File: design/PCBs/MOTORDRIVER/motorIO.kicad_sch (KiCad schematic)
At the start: 3 parts, among them J5 1-84952-1, J6 1-84952-1, J7 1-84952-1

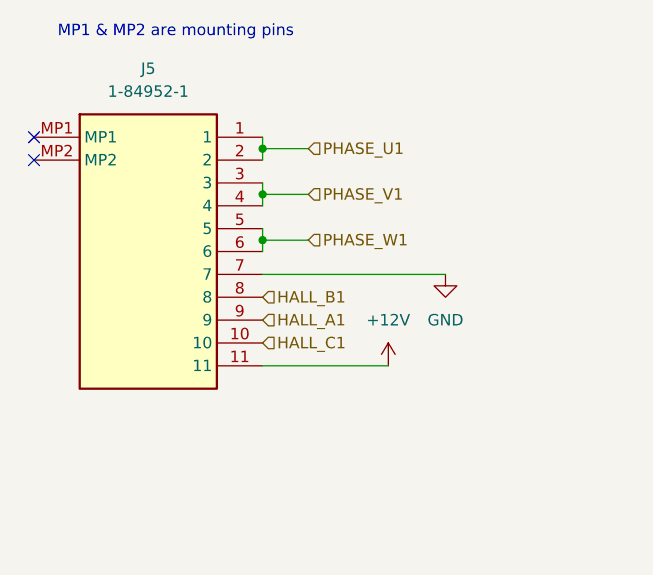
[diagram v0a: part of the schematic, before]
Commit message: worked on schemtaic
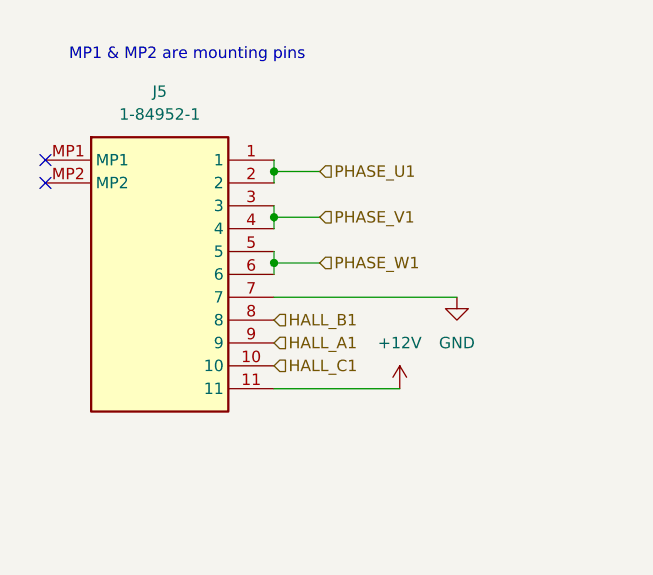
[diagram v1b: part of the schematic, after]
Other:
- moved on the sheet: J5
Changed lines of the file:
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@@
 	)
 	(junction
-		(at 82.55 102.87)
+		(at 83.82 105.41)
 		(diameter 0)
 		(color 0 0 0 0)
@@
 	)
 	(junction
-		(at 82.55 92.71)
+		(at 83.82 95.25)
 		(diameter 0)
 		(color 0 0 0 0)
@@
 	)
 	(junction
-		(at 82.55 97.79)
+		(at 83.82 100.33)
 		(diameter 0)
 		(color 0 0 0 0)
@@
 	)
 	(no_connect
-		(at 57.15 91.44)
+		(at 58.42 93.98)
 	)
 	(no_connect
-		(at 57.15 93.98)
+		(at 58.42 96.52)
 	)
 	(no_connect
@@
 	(wire
 		(pts
-			(xy 87.63 102.87) (xy 82.55 102.87)
+			(xy 88.9 105.41) (xy 83.82 105.41)
 		)
 		(stroke
@@
 	(wire
 		(pts
-			(xy 82.55 97.79) (xy 82.55 99.06)
+			(xy 83.82 100.33) (xy 83.82 101.6)
 		)
 		(stroke
@@
 	(wire
 		(pts
-			(xy 87.63 92.71) (xy 82.55 92.71)
+			(xy 88.9 95.25) (xy 83.82 95.25)
 		)
 		(stroke
@@
 	(wire
 		(pts
-			(xy 82.55 101.6) (xy 82.55 102.87)
+			(xy 83.82 104.14) (xy 83.82 105.41)
 		)
 		(stroke
@@
 	(wire
 		(pts
-			(xy 87.63 97.79) (xy 82.55 97.79)
+			(xy 88.9 100.33) (xy 83.82 100.33)
 		)
 		(stroke
@@
 	(wire
 		(pts
-			(xy 96.52 116.84) (xy 82.55 116.84)
-		)
-		(stroke
-			(width 0)
-			(type default)
-		)
-	)
-	(wire
-		(pts
-			(xy 82.55 102.87) (xy 82.55 104.14)
+			(xy 97.79 119.38) (xy 83.82 119.38)
+		)
+		(stroke
+			(width 0)
+			(type default)
+		)
+	)
+	(wire
+		(pts
+			(xy 83.82 105.41) (xy 83.82 106.68)
 		)
 		(stroke
@@
 	(wire
 		(pts
-			(xy 82.55 91.44) (xy 82.55 92.71)
+			(xy 83.82 93.98) (xy 83.82 95.25)
 		)
 		(stroke
@@
 	(wire
 		(pts
-			(xy 82.55 106.68) (xy 102.87 106.68)
+			(xy 83.82 109.22) (xy 104.14 109.22)
 		)
 		(stroke
@@
 	(wire
 		(pts
-			(xy 82.55 92.71) (xy 82.55 93.98)
-		)
-		(stroke
-			(width 0)
-			(type default)
-		)
-	)
-	(wire
-		(pts
-			(xy 82.55 96.52) (xy 82.55 97.79)
+			(xy 83.82 95.25) (xy 83.82 96.52)
+		)
+		(stroke
+			(width 0)
+			(type default)
+		)
+	)
+	(wire
+		(pts
+			(xy 83.82 99.06) (xy 83.82 100.33)
 		)
 		(stroke
@@
 	(text "MP1 & MP2 are mounting pins"
 		(exclude_from_sim no)
-		(at 72.898 79.756 0)
+		(at 74.168 82.296 0)
 		(effects
 			(font
@@
 	(hierarchical_label "PHASE_W1"
 		(shape input)
-		(at 87.63 102.87 0)
+		(at 88.9 105.41 0)
 		(fields_autoplaced yes)
 		(effects
@@
 	(hierarchical_label "HALL_B1"
 		(shape input)
-		(at 82.55 109.22 0)
+		(at 83.82 111.76 0)
 		(fields_autoplaced yes)
 		(effects
@@
 	(hierarchical_label "PHASE_V1"
 		(shape input)
-		(at 87.63 97.79 0)
+		(at 88.9 100.33 0)
 		(fields_autoplaced yes)
 		(effects
@@
 	(hierarchical_label "PHASE_U1"
 		(shape input)
-		(at 87.63 92.71 0)
+		(at 88.9 95.25 0)
 		(fields_autoplaced yes)
 		(effects
@@
 	(hierarchical_label "HALL_A1"
 		(shape input)
-		(at 82.55 111.76 0)
+		(at 83.82 114.3 0)
 		(fields_autoplaced yes)
 		(effects
@@
 	(hierarchical_label "HALL_C1"
 		(shape input)
-		(at 82.55 114.3 0)
+		(at 83.82 116.84 0)
 		(fields_autoplaced yes)
 		(effects
@@
 	(symbol
 		(lib_id "power:+12V")
-		(at 96.52 116.84 0)
+		(at 97.79 119.38 0)
 		(unit 1)
 		(exclude_from_sim no)
@@
 		(fields_autoplaced yes)
 		(property "Reference" "#PWR0208"
-			(at 96.52 120.65 0)
+			(at 97.79 123.19 0)
 			(effects
 				(font
@@
 		)
 		(property "Value" "+12V"
-			(at 96.52 111.76 0)
+			(at 97.79 114.3 0)
 			(effects
 				(font
@@
 		)
 		(property "Footprint" ""
-			(at 96.52 116.84 0)
+			(at 97.79 119.38 0)
 			(effects
 				(font
@@
 		)
 		(property "Datasheet" ""
-			(at 96.52 116.84 0)
+			(at 97.79 119.38 0)
 			(effects
 				(font
@@
 		)
 		(property "Description" "Power symbol creates a global label with name \"+12V\""
-			(at 96.52 116.84 0)
+			(at 97.79 119.38 0)
 			(effects
 				(font
@@
 	(symbol
 		(lib_id "power:GND")
-		(at 102.87 106.68 0)
+		(at 104.14 109.22 0)
 		(unit 1)
 		(exclude_from_sim no)
@@
 		(fields_autoplaced yes)
 		(property "Reference" "#PWR0209"
-			(at 102.87 113.03 0)
+			(at 104.14 115.57 0)
 			(effects
 				(font
@@
 		)
 		(property "Value" "GND"
-			(at 102.87 111.76 0)
+			(at 104.14 114.3 0)
 			(effects
 				(font
@@
 		)
 		(property "Footprint" ""
-			(at 102.87 106.68 0)
+			(at 104.14 109.22 0)
 			(effects
 				(font
@@
 		)
 		(property "Datasheet" ""
-			(at 102.87 106.68 0)
+			(at 104.14 109.22 0)
 			(effects
 				(font
@@
 		)
 		(property "Description" "Power symbol creates a global label with name \"GND\" , ground"
-			(at 102.87 106.68 0)
+			(at 104.14 109.22 0)
 			(effects
 				(font
@@
 	(symbol
 		(lib_id "1-84952-1:1-84952-1")
-		(at 57.15 91.44 0)
+		(at 58.42 93.98 0)
 		(unit 1)
 		(exclude_from_sim no)
@@
 		(fields_autoplaced yes)
 		(property "Reference" "J5"
-			(at 69.85 83.82 0)
+			(at 71.12 86.36 0)
 			(effects
 				(font
@@
 		)
 		(property "Value" "1-84952-1"
-			(at 69.85 86.36 0)
+			(at 71.12 88.9 0)
 			(effects
 				(font
@@
 		)
 		(property "Footprint" "kuben-footprints:1849521"
-			(at 78.74 186.36 0)
+			(at 80.01 188.9 0)
 			(effects
 				(font
@@
 		)
 		(property "Datasheet" "https://componentsearchengine.com/Datasheets/2/1-84952-1.pdf"
-			(at 78.74 286.36 0)
+			(at 80.01 288.9 0)
 			(effects
 				(font
@@
 		)
 		(property "Description" "FFC & FPC Connectors 1MM FPC HORZ .BTTM CONT.ASS.11P"
-			(at 57.15 91.44 0)
+			(at 58.42 93.98 0)
 			(effects
 				(font
@@
 		)
 		(property "Height" "2.74"
-			(at 78.74 486.36 0)
+			(at 80.01 488.9 0)
 			(effects
 				(font
@@
 		)
 		(property "Mouser Part Number" "571-1-84952-1"
-			(at 78.74 586.36 0)
+			(at 80.01 588.9 0)
 			(effects
 				(font
@@
 		)
 		(property "Mouser Price/Stock" "https://www.mouser.co.uk/ProductDetail/TE-Connectivity/1-84952-1?qs=uUkeXfjQ8uS9Vjbveobf0Q%3D%3D"
-			(at 78.74 686.36 0)
+			(at 80.01 688.9 0)
 			(effects
 				(font
@@
 		)
 		(property "Manufacturer_Name" "TE Connectivity"
-			(at 78.74 786.36 0)
+			(at 80.01 788.9 0)
 			(effects
 				(font
@@
 		)
 		(property "Manufacturer_Part_Number" "1-84952-1"
-			(at 78.74 886.36 0)
-			(effects
-				(font
+			(at 80.01 888.9 0)
+			(effects
+				(font
